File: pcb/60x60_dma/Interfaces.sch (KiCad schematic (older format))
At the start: 18 parts, among them J1 Conn_01x05, J10 Conn_01x01_Female, J11 Conn_01x01_Female, J12 Conn_01x01_Female, J13 Conn_01x01_Female, J14 Conn_01x02, J15 Conn_01x04, J2 Conn_01x05, J3 USB_OTG, J4 Conn_01x05, J5 Conn_01x05, J6 Conn_01x05, J7 Conn_01x05, J8 Conn_01x05, J9 Conn_01x05, Q2 IRLML6402

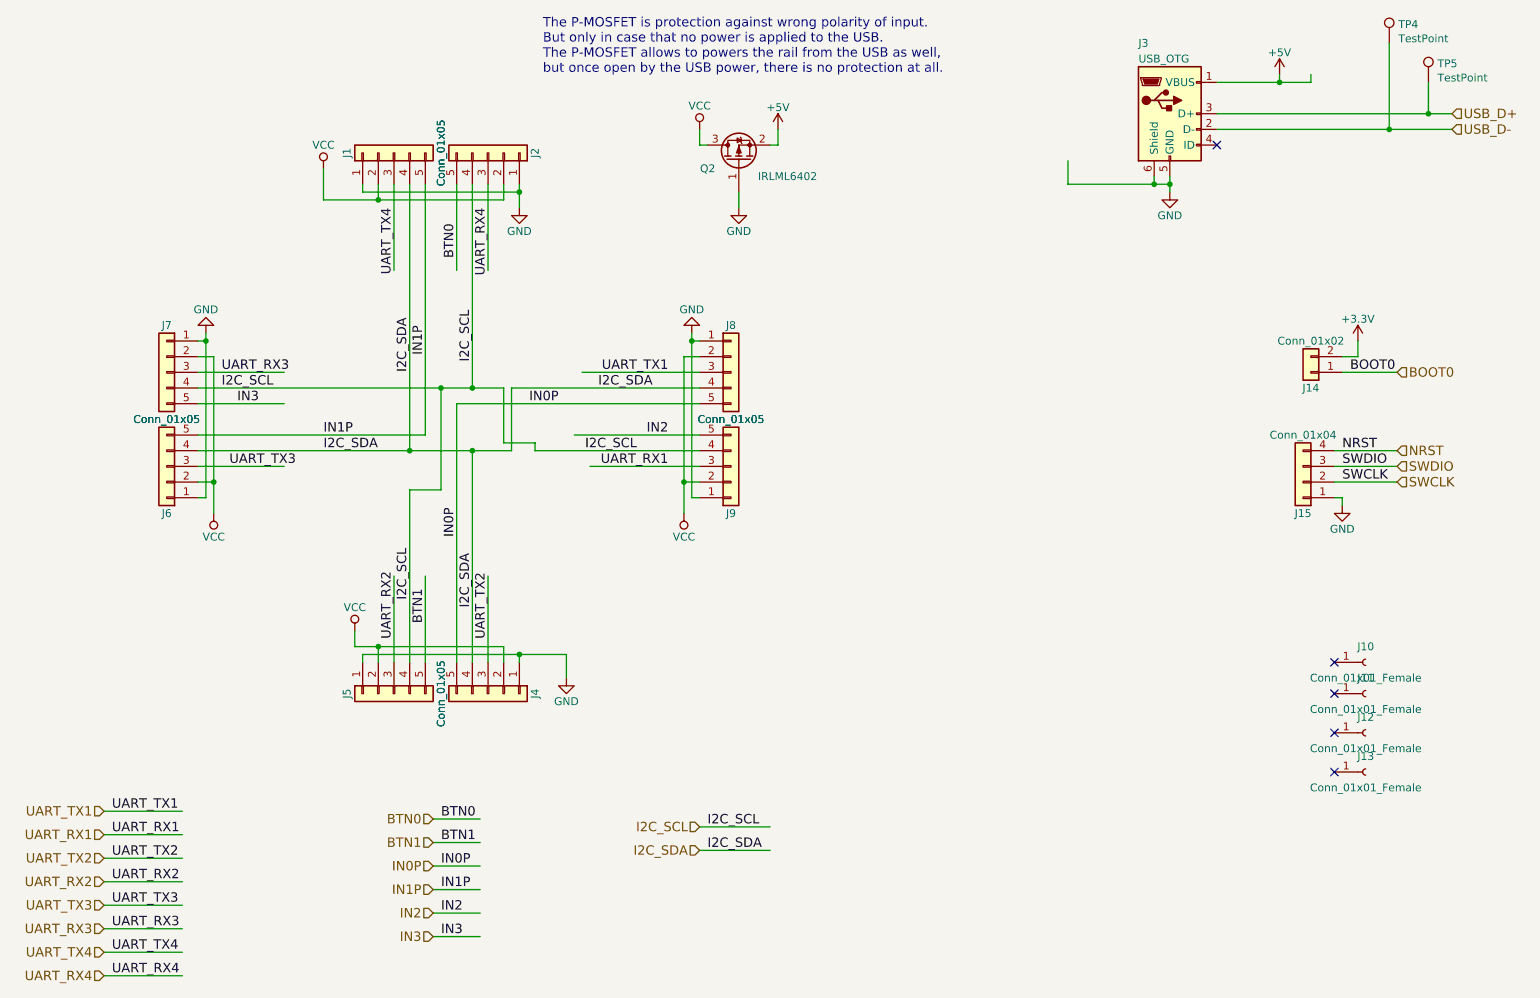
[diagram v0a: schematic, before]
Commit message: - clense the schematics
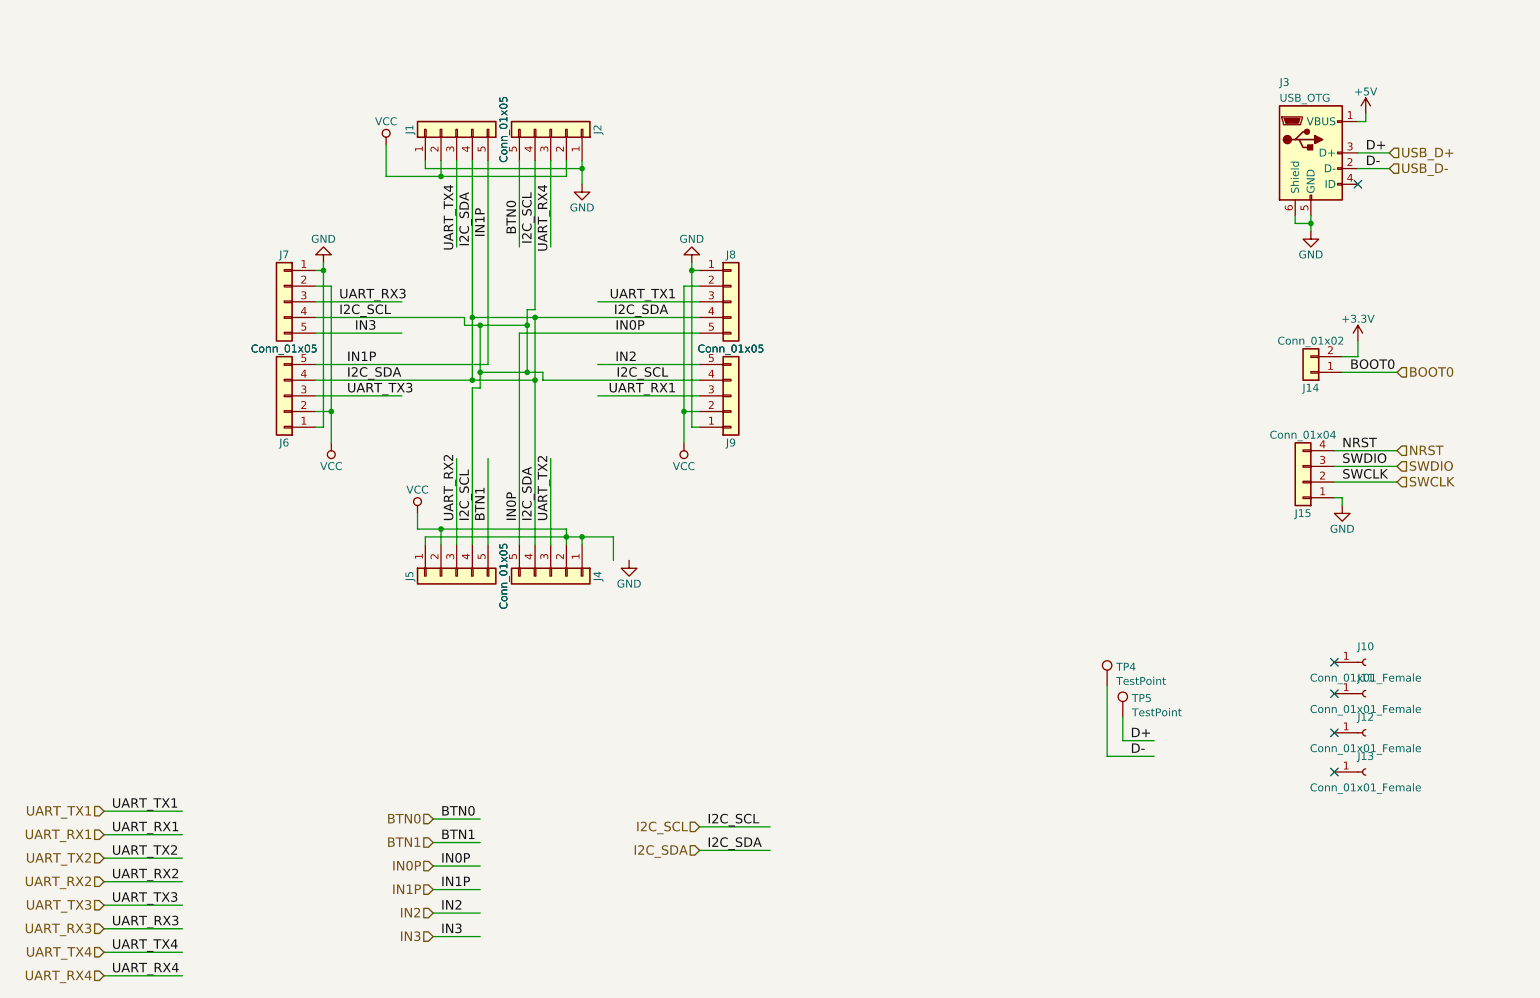
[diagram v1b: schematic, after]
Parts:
- removed Q2: IRLML6402, kicad_libraries_new:badger_SOT-23_handsolder, symbol bcl4v2-rescue:Q_PMOS_GSD
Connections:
- net labels added: D+, D-
- wire segments 114 -> 113
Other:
- note removed: "The P-MOSFET is protection against wrong polarity of input.\nBut only in case that no power is applied to the USB.\nThe P-MOSFET allows to powers the rail from the USB as well,\nbut once open by the USB power, there is no protection at all."
- moved on the sheet: J1, J2, J3, J4, J5, J6, J7, J8, J9, TP4, TP5
